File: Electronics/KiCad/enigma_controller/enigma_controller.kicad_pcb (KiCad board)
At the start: 6 copper layers, 227.9 x 120.8 mm, 77 parts, among them IC1 SN74LVC257ADR, IC10 MCP23017-E_SO, IC11 RT9742SNGV, IC2 SN74LVC257ADR, IC3 SN74LVC257ADR, IC4 SN74LVC257ADR, IC5 SN74LVC257ADR, IC6 SN74LVC257ADR, IC7 SN74LVC257ADR, IC8 AP22653W6-7, IC9 MCP23017-E_SO, J1 Conn_02x07_Odd_Even, J10 0936263006, J11 Conn_02x05_Odd_Even, J14 USB_C_Receptacle_PowerOnly_6P, J15 Conn_01x02, J16 Conn_01x02, J17 Conn_01x02, J18 Conn_01x02, J19 Conn_01x02, J2 Conn_02x07_Odd_Even, J20 Conn_01x02, J21 Conn_02x05_Odd_Even, J22 Conn_02x05_Odd_Even, J23 Conn_01x02, J24 Conn_01x02, J25 Conn_01x02, J26 Conn_01x02, J27 Conn_01x02, J28 Conn_02x03_Odd_Even, J3 USB1040-GF-L-B, J5 46765-0301, J6 Conn_02x05_Odd_Even, J7 Conn_02x07_Odd_Even, J8 USB3_A_Stacked, J9 Conn_02x07_Odd_Even, M1 Fan_4pin

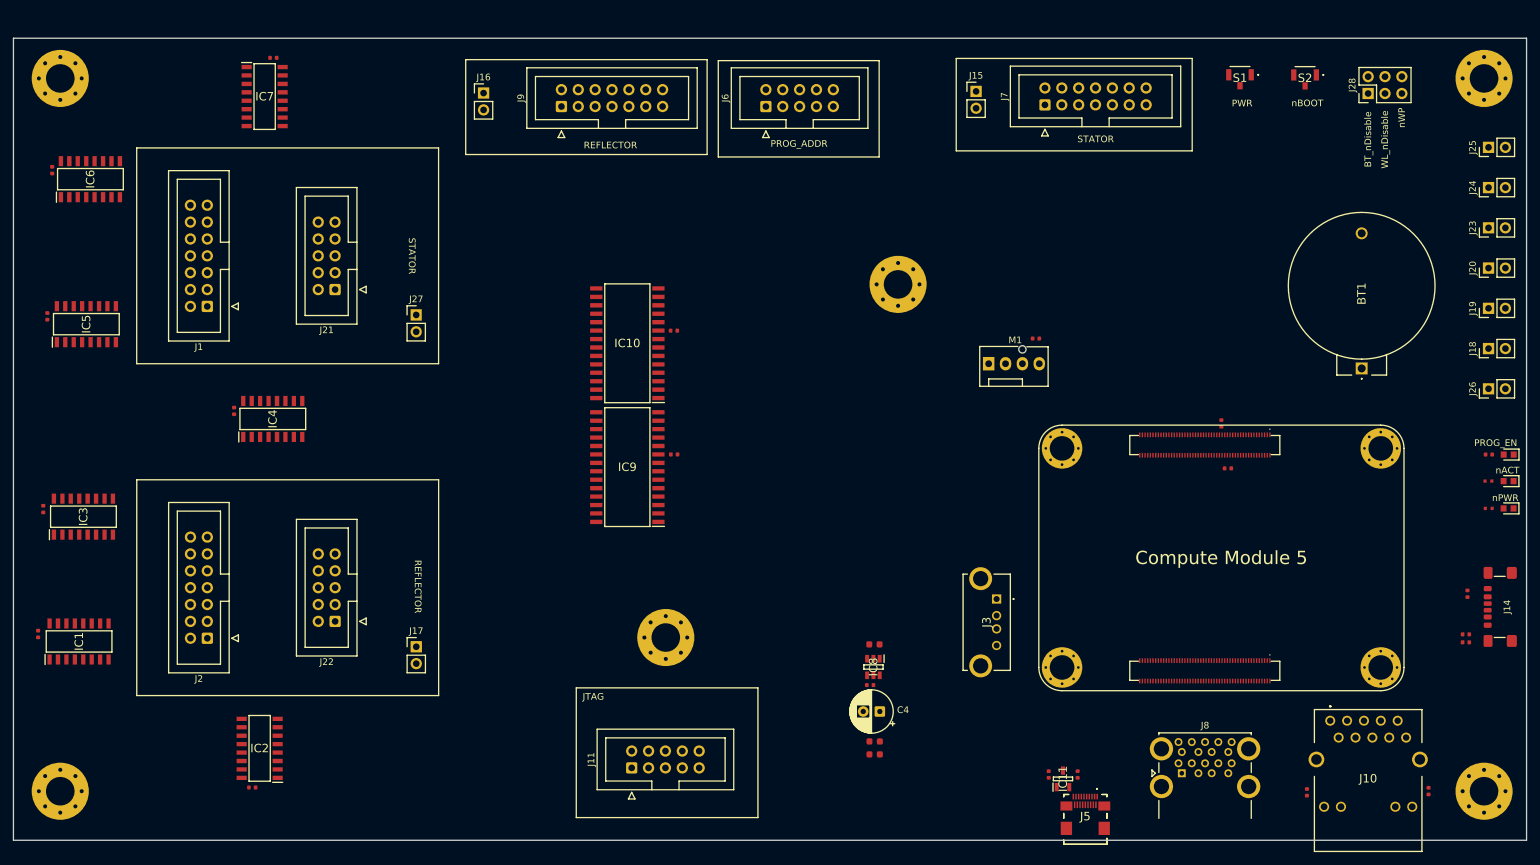
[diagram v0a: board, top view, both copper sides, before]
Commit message: PCB Layout [AS-Review-1]
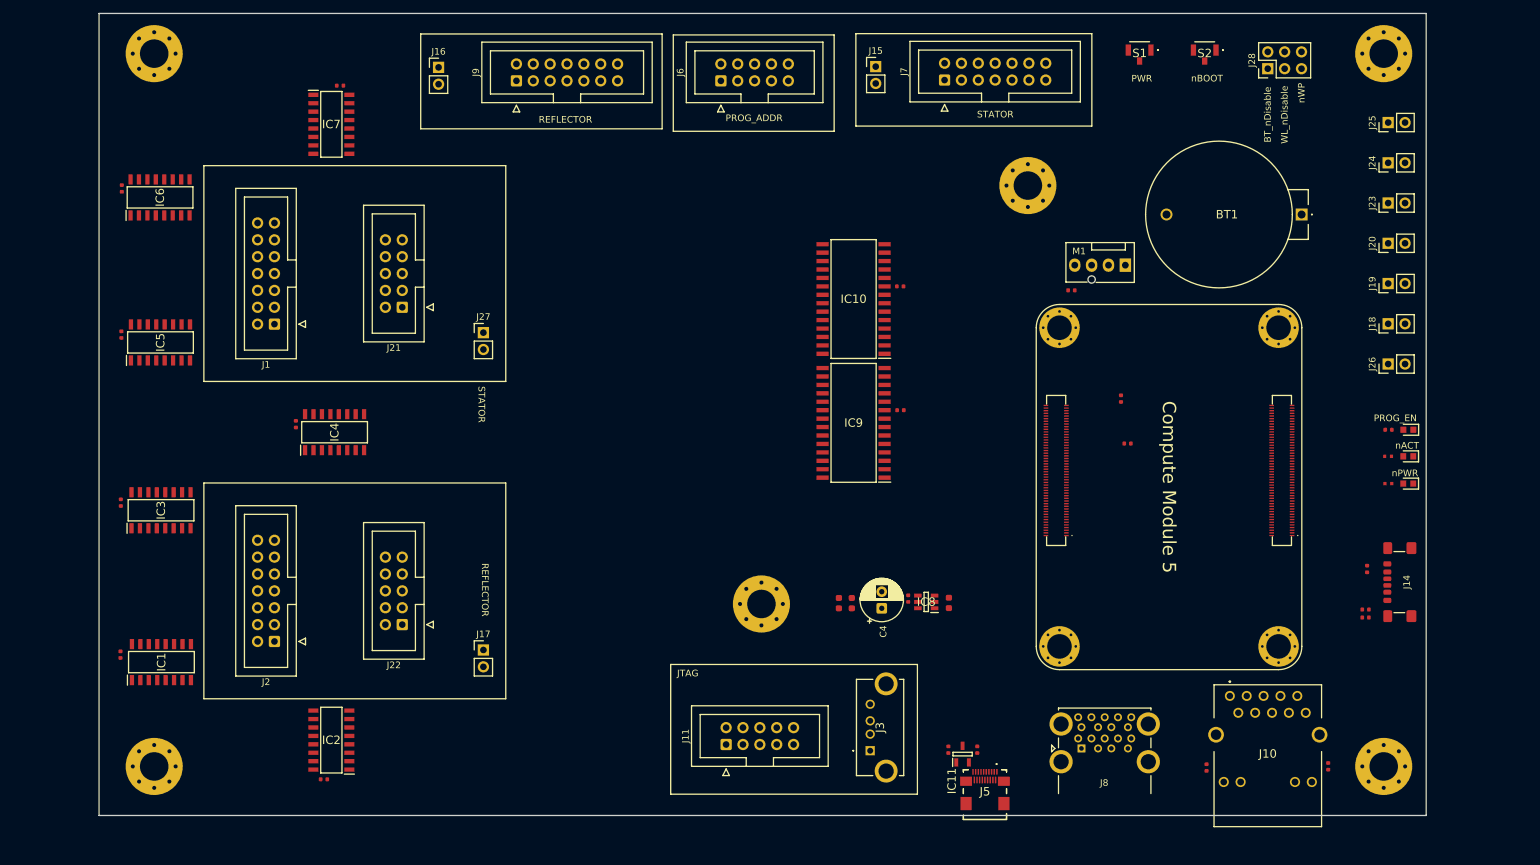
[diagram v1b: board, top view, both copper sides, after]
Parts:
- moved H1 41.8 mm to (190.3, 93.7), turned to -90 degrees
- moved C17 34.7 mm to (169.9, 84.6)
- moved IC10 34.7 mm to (162.8, 67.9)
- moved IC9 34.7 mm to (162.8, 86.5)
- moved C13 34.7 mm to (169.8, 66.0)
- moved J3 29.7 mm to (165.3, 135.9), turned to 90 degrees
- moved M1 25.4 mm to (203.7, 62.8), turned to 180 degrees
- moved BT1 24.9 mm to (230.3, 55.2), turned to 0 degrees
- moved H7 24.6 mm to (189.1, 50.8)
- moved C3 23.4 mm to (160.6, 113.7), turned to 90 degrees
- moved C19 21.1 mm to (162.5, 113.7), turned to 90 degrees
- moved H4 15.6 mm to (242.6, 30.9)
- moved LED2 15.6 mm to (246.3, 95.7)
- moved S1 15.6 mm to (205.9, 30.4)
- moved H6 15.6 mm to (242.6, 138.3)
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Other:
- board size 227.9 x 120.8 mm -> 199.9 x 120.8 mm
